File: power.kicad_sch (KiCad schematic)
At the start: 4 parts, among them J1 USB_C_Receptacle_USB2.0_16P, U2 USBLC6-2SC6

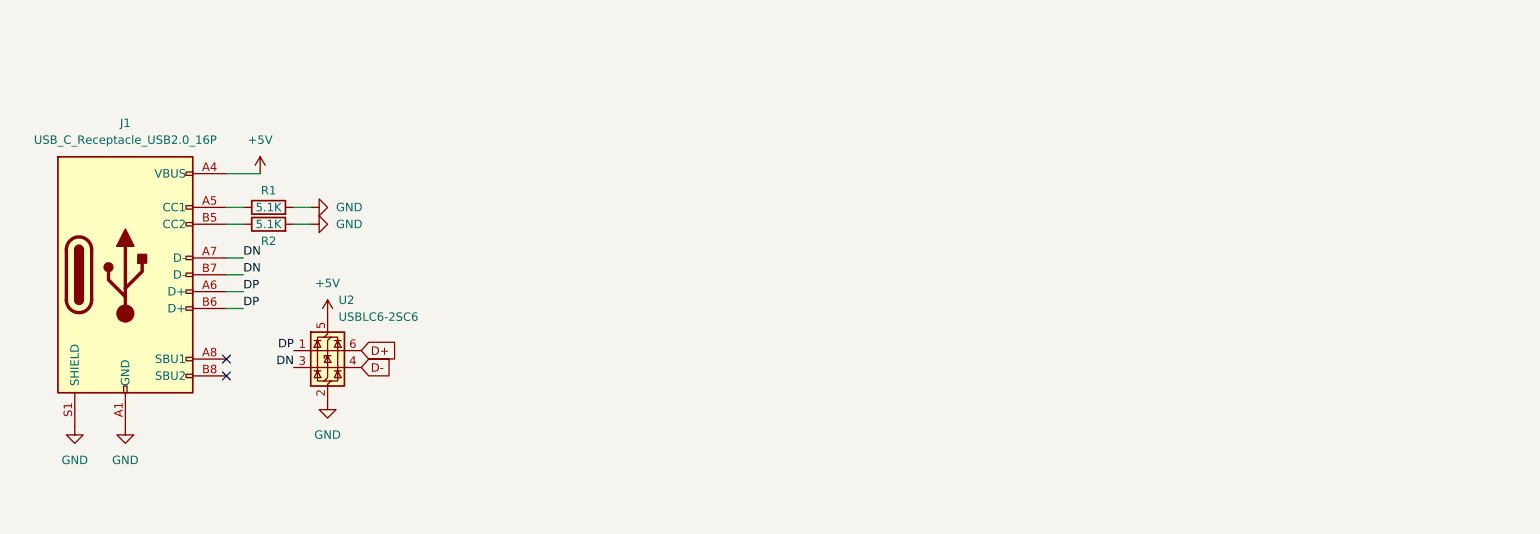
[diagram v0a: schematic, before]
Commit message: add power
Signed-off-by: HaoboGu <haobogu@outlook.com>
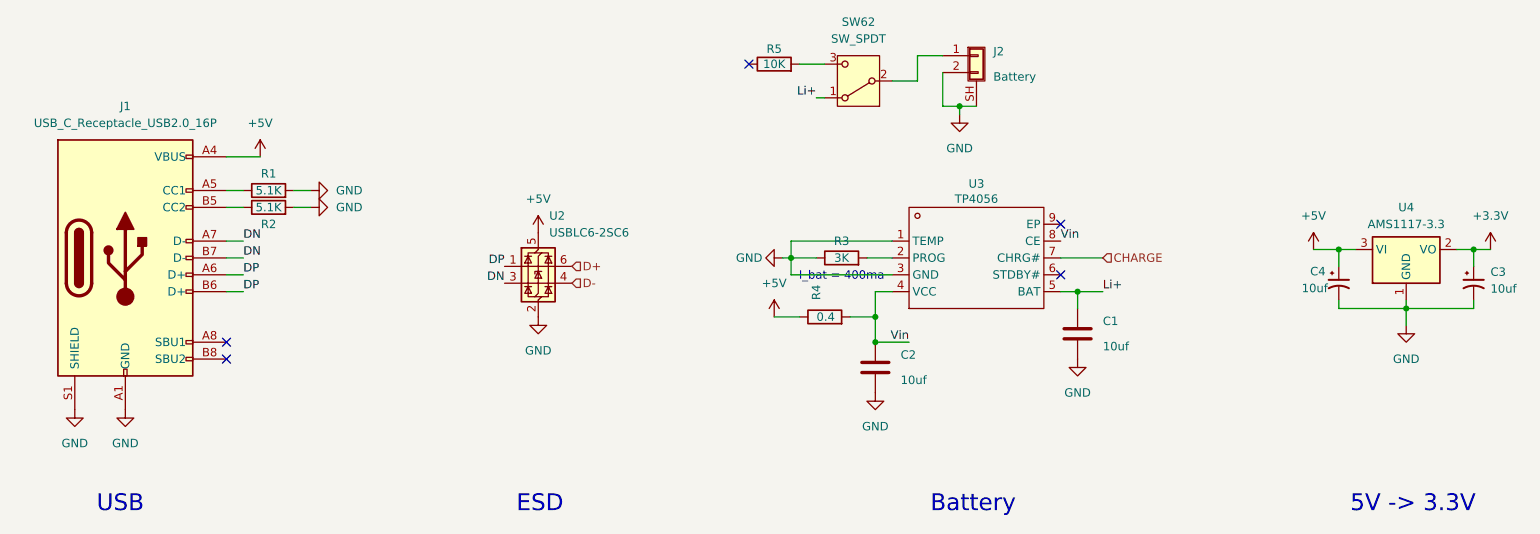
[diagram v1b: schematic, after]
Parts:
- added C1, C2: 10uf, symbol Device:C
- added C3, C4: 10uf, symbol Device:C_Polarized_Small_US
- added J2: Battery, Connector_JST:JST_SH_SM02B-SRSS-TB_1x02-1MP_P1.00mm_Horizontal, symbol Connector_Generic_Shielded:Conn_01x02_Shielded
- added R3: 3K, symbol Device:R
- added R4: 0.4, symbol Device:R
- added R5: 10K, symbol Device:R
- added SW62: SW_SPDT, symbol Switch:SW_SPDT
- added U3: TP4056, TP4056:ESOP-8_L4.9-W3.9-P1.27-LS6.0-BL-EP, symbol TP4056:TP4056_C725790
- added U4: AMS1117-3.3, Package_TO_SOT_SMD:SOT-223-3_TabPin2, symbol Regulator_Linear:AMS1117-3.3
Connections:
- net +5V: now also C4.1, R4.1, U4.3 (VI)
- net GND: now also C1.2, C2.2, C3.2, C4.2, J2.2 (Pin_2), J2.SH (Shield), R3.1, U3.1 (TEMP), U3.3 (GND), U4.1 (GND)
- new net: J2.1 (Pin_1), SW62.2 (B)
- new net: R5.2, SW62.3 (C)
- new net: R3.2, U3.2 (PROG)
- new net +3.3V: C3.1, U4.2 (VO)
- new net CHARGE: U3.7 (CHRG#)
- new net Li+: C1.1, SW62.1 (A), U3.5 (BAT)
- new net Vin: C2.1, R4.2, U3.4 (VCC), U3.8 (CE)
- no-connect marks 2 -> 5
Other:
- note added: "5V -> 3.3V"
- note added: "Battery"
- note added: "ESD"
- note added: "I_bat = 400ma"
- note added: "USB"
- moved on the sheet: J1, R1, R2, U2
